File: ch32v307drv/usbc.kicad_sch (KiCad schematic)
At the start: 7 parts, among them J2 Connector, USB-TYPE-C-16P, U3 CH221K

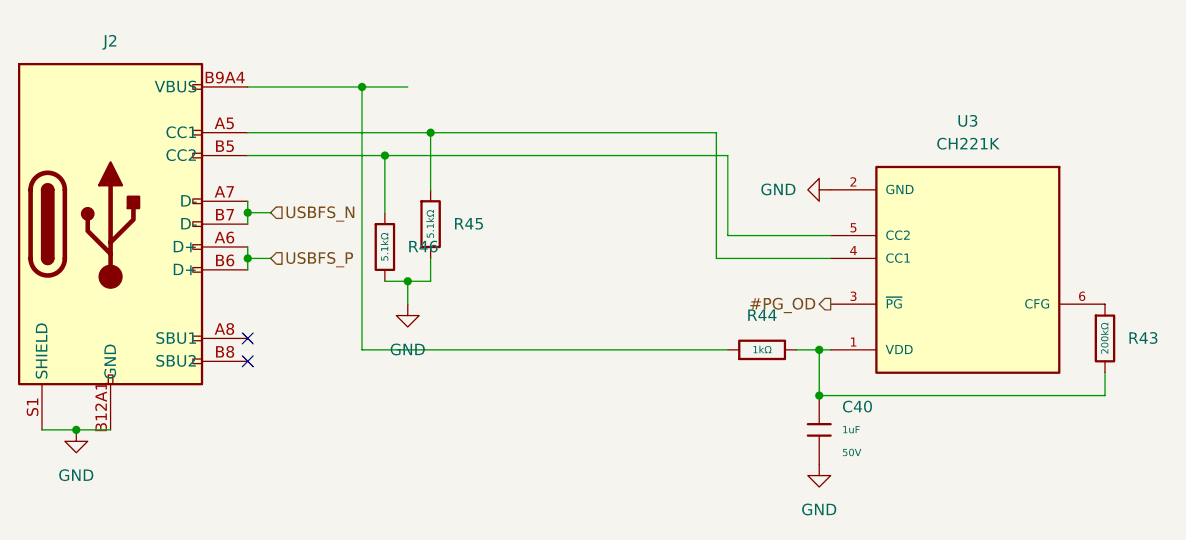
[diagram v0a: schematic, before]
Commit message: more design
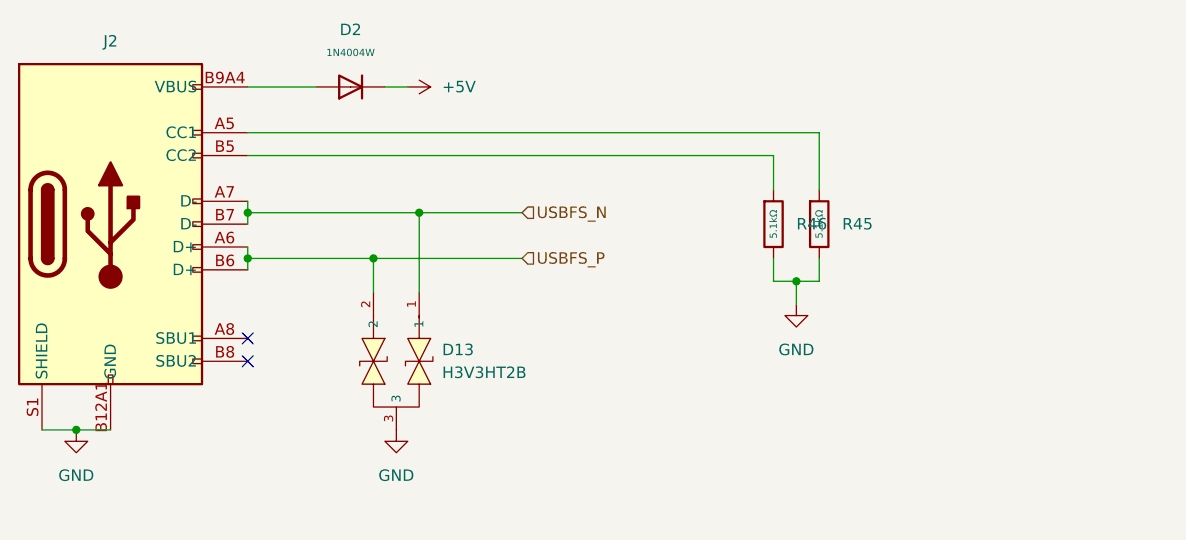
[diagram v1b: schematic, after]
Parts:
- removed C40: 1uF, PCM_JLCPCB:C_0603, symbol PCM_JLCPCB-Capacitors:0603,1uF
- removed R43: 200kΩ, PCM_JLCPCB:R_0603, symbol PCM_JLCPCB-Resistors:0603,200kΩ
- removed R44: 1kΩ, PCM_JLCPCB:R_0603, symbol PCM_JLCPCB-Resistors:0603,1kΩ
- removed U3: CH221K, CH221K:SOT95P280X120-6N, symbol CH221K:CH221K
- added D13: H3V3HT2B, PCM_JLCPCB:SOT-23-3_L2.9-W1.3-P1.90-LS2.4-BR, symbol PCM_JLCPCB-Diode-Packages:TVS-Bi, H3V3HT2B
- added D2: 1N4004W, PCM_JLCPCB:D_SOD-123FL, symbol PCM_JLCPCB-Diodes:General,1N4004W
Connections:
- net GND: now also D13.3
- net USBFS_N: now also D13.1
- net USBFS_P: now also D13.2
- net at J2.A9B4 (VBUS), J2.B9A4 (VBUS): now also D2.2
- new net +5V: D2.1
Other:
- moved on the sheet: R45, R46
